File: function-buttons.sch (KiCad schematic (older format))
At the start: 74 parts, among them Q1 MMBT3904, Q10 MMBT3904, Q2 MMBT3904, Q3 MMBT3904, Q4 MMBT3904, Q5 MMBT3904, Q6 MMBT3904, Q7 MMBT3904, Q8 MMBT3904, Q9 MMBT3904, SW1 SHIFT, SW10 ADDR_SAFE_AREA, SW2 HORIZ_SYNC, SW3 UNDERSCAN_16_9, SW4 VERT_BLUE_ONLY, SW5 MONO_R, SW6 APT_G, SW7 COMB_B, SW8 F1_F3, SW9 F2_F4, U14 74LVC2G14, U15 74LVC2G14, U2 74HC14

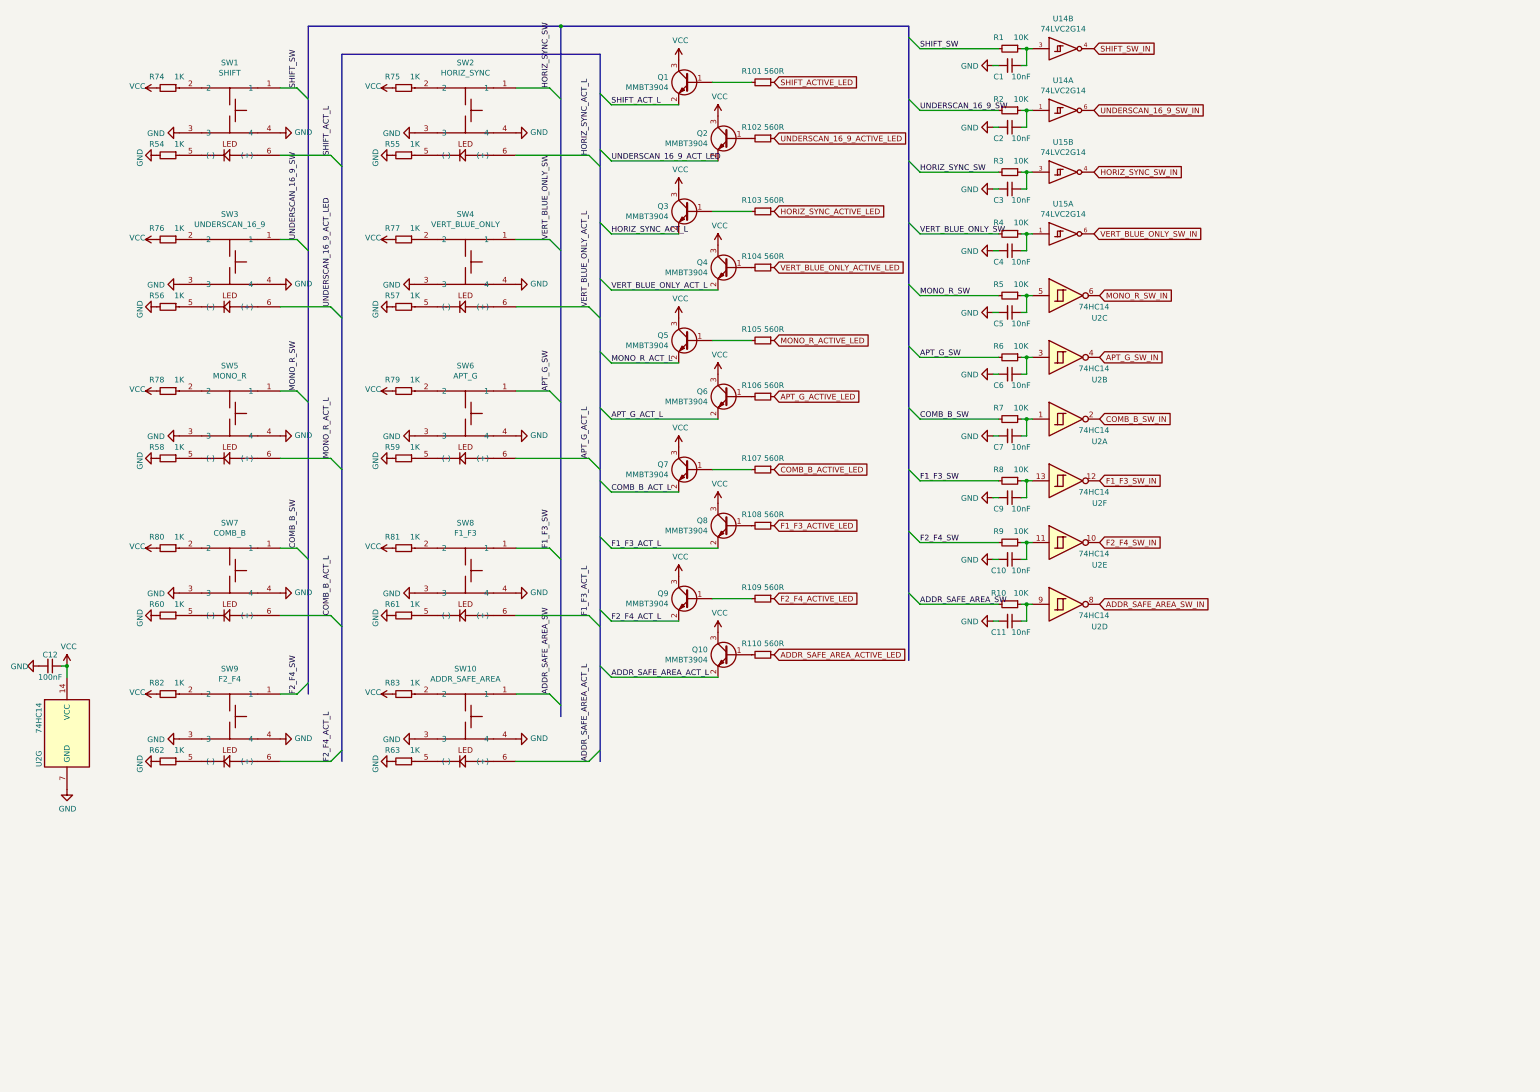
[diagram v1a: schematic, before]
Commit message: Initial revision B
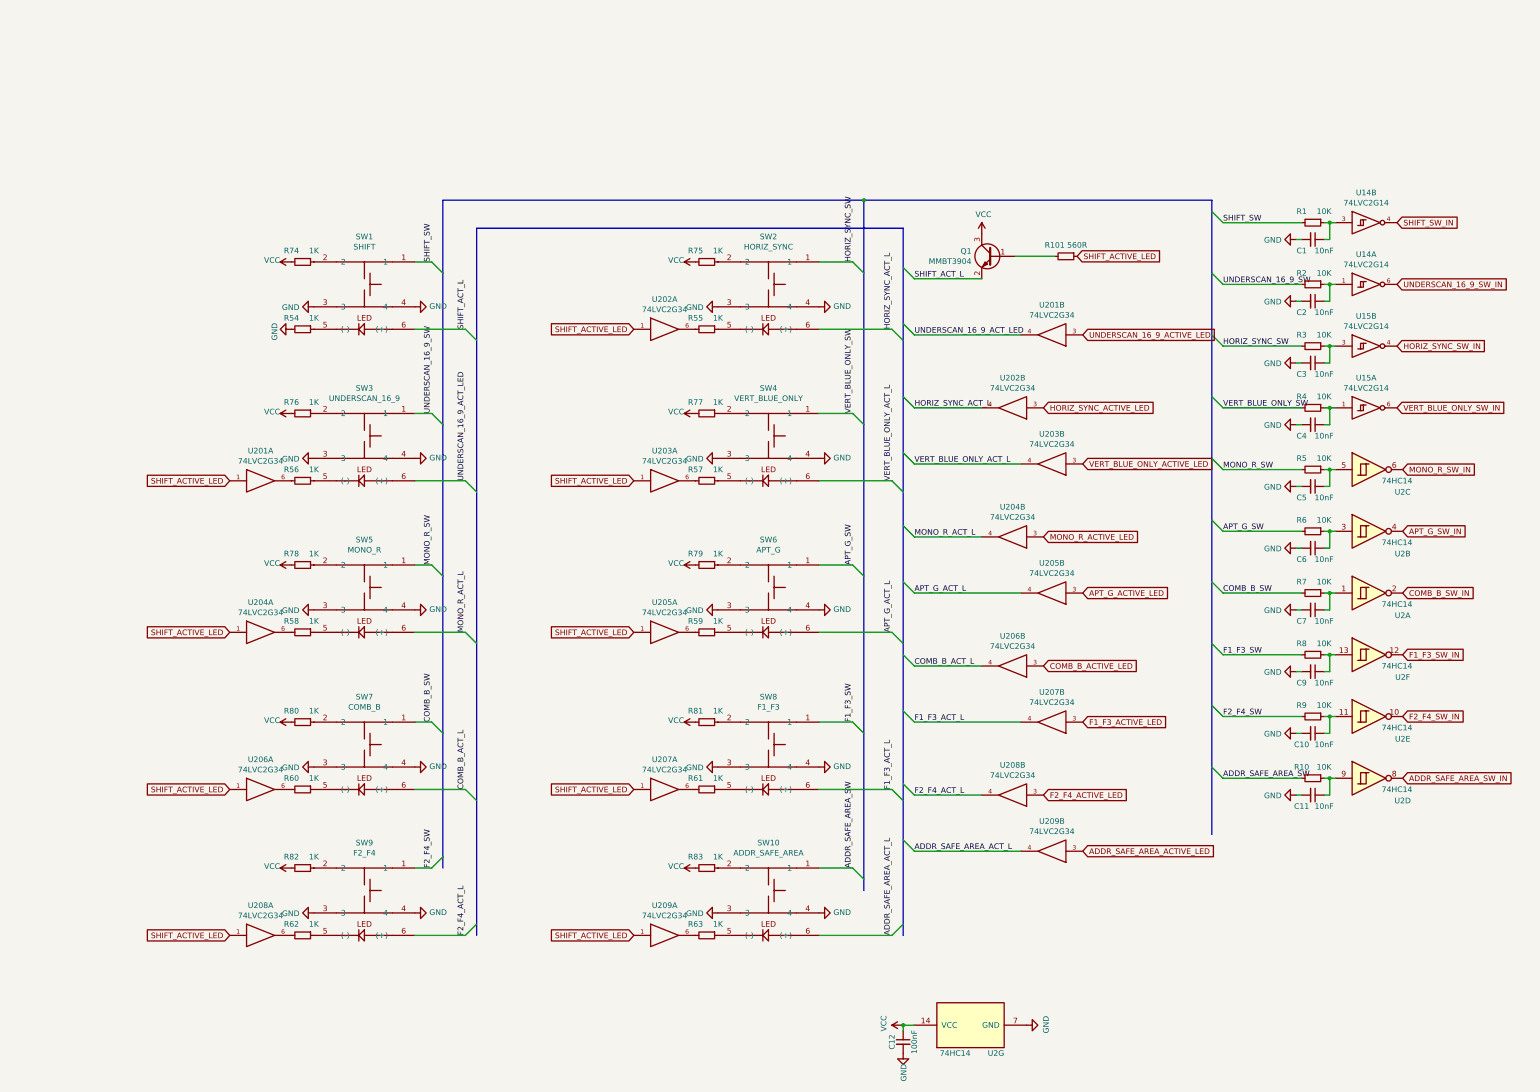
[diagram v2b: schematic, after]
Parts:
- removed Q10, Q2, Q3, Q4, Q5, Q6, Q7, Q8, Q9: MMBT3904, Package_TO_SOT_SMD:SOT-23, symbol Transistor_BJT:MMBT3904
- removed R102, R103, R104, R105, R106, R107, R108, R109, R110: 560R, Resistor_SMD:R_0603_1608Metric_Pad0.98x0.95mm_HandSolder, symbol Device:R_Small
- added U201, U202, U203, U204, U205, U206, U207, U208, U209: 74LVC2G34, Package_TO_SOT_SMD:SOT-23-6_Handsoldering, symbol 74xGxx:74LVC2G34
- SW1, SW10, SW2, SW3, SW4, SW5, SW6, SW7, SW8, SW9: footprint TL-1240:TL-1240 -> TL-1265:TL-1265
- U2: footprint Package_SO:SSOP-14_5.3x6.2mm_P0.65mm -> Package_SO:TSSOP-14_4.4x5mm_P0.65mm
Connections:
- net ADDR_SAFE_AREA_ACTIVE_LED: now also U209.3
- net ADDR_SAFE_AREA_ACT_L: now also U209.4
- net APT_G_ACTIVE_LED: now also U205.3
- net APT_G_ACT_L: now also U205.4
- net COMB_B_ACTIVE_LED: now also U206.3
- net COMB_B_ACT_L: now also U206.4
- net F1_F3_ACTIVE_LED: now also U207.3
- net F1_F3_ACT_L: now also U207.4
- net F2_F4_ACTIVE_LED: now also U208.3
- net F2_F4_ACT_L: now also U208.4
- net GND: now also U201.2 (GND), U201.2 (GND), U202.2 (GND), U202.2 (GND), U203.2 (GND), U203.2 (GND), U204.2 (GND), U204.2 (GND), U205.2 (GND), U205.2 (GND), U206.2 (GND), U206.2 (GND), U207.2 (GND), U207.2 (GND), U208.2 (GND), U208.2 (GND), U209.2 (GND), U209.2 (GND); no longer R55.2, R56.2, R57.2, R58.2, R59.2, R60.2, R61.2, R62.2, R63.2
- net HORIZ_SYNC_ACTIVE_LED: now also U202.3
- net HORIZ_SYNC_ACT_L: now also U202.4
- net MONO_R_ACTIVE_LED: now also U204.3
- net MONO_R_ACT_L: now also U204.4
- net SHIFT_ACTIVE_LED: now also U201.1, U202.1, U203.1, U204.1, U205.1, U206.1, U207.1, U208.1, U209.1
- net UNDERSCAN_16_9_ACTIVE_LED: now also U201.3
- net UNDERSCAN_16_9_ACT_LED: now also U201.4
- net VCC: now also U201.5 (VCC), U201.5 (VCC), U202.5 (VCC), U202.5 (VCC), U203.5 (VCC), U203.5 (VCC), U204.5 (VCC), U204.5 (VCC), U205.5 (VCC), U205.5 (VCC), U206.5 (VCC), U206.5 (VCC), U207.5 (VCC), U207.5 (VCC), U208.5 (VCC), U208.5 (VCC), U209.5 (VCC), U209.5 (VCC)
- net VERT_BLUE_ONLY_ACTIVE_LED: now also U203.3
- net VERT_BLUE_ONLY_ACT_L: now also U203.4
- new net: R56.2, U201.6
- new net: R58.2, U204.6
- new net: R60.2, U206.6
- new net: R62.2, U208.6
- new net: R55.2, U202.6
- new net: R57.2, U203.6
- new net: R59.2, U205.6
- new net: R61.2, U207.6
- new net: R63.2, U209.6
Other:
- moved on the sheet: C1, C10, C11, C12, C2, C3, C4, C5, C6, C7, C9, Q1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
